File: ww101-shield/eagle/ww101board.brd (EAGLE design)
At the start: 64.8 x 73.3 mm, 66 parts, among them J6 U8G-096-OLED, J7 0, U7 CY8C4A45-48

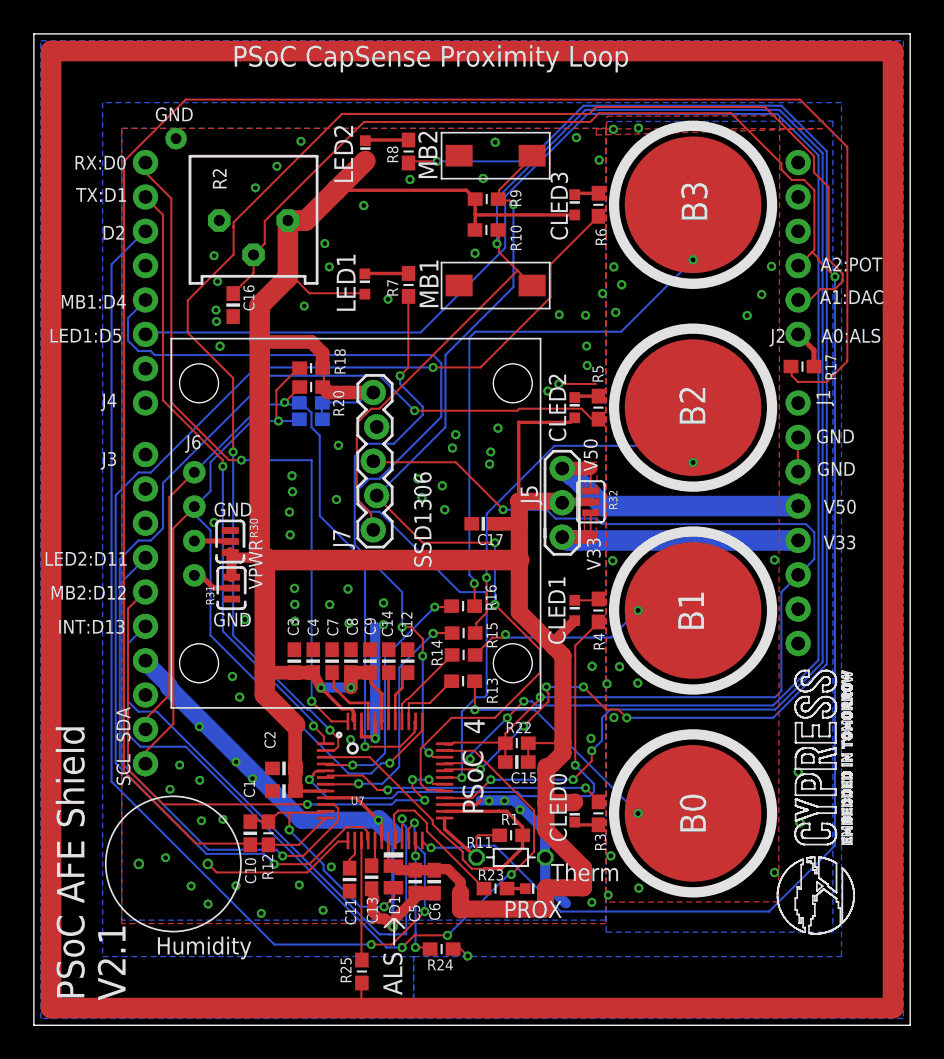
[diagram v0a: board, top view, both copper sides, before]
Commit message: a bunch of updates
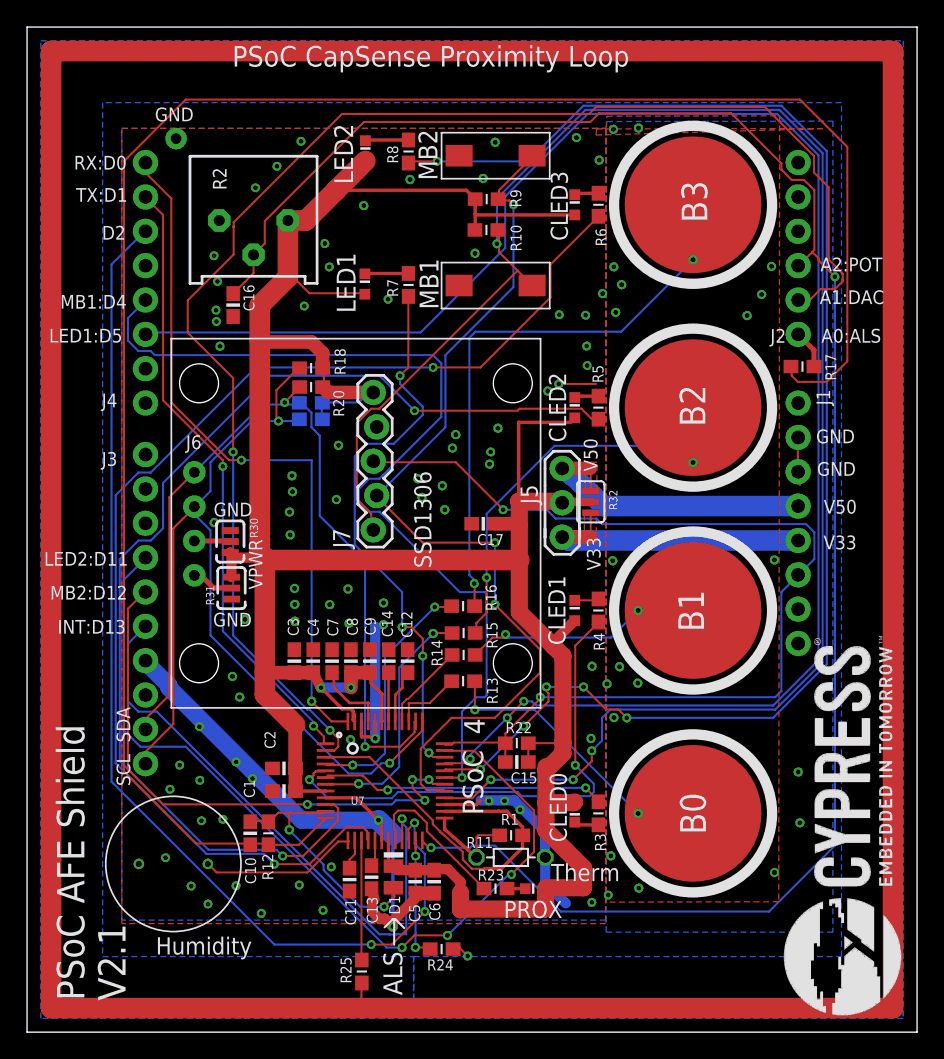
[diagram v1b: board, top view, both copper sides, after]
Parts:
- removed U$3: (no value), IOTExpert:CYPRESSLOGO
- added U$7: CYLOGO-SILK, ww101board:CYLOGO-SILK
- R18, R19, R20, R21: value 4.7K -> DNP
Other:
- board size 64.8 x 73.3 mm -> 65.8 x 74.3 mm
- board text added: "600-60500-01 REV2.1"
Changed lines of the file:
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@@
 <layer number="17" name="Pads" color="2" fill="1" visible="yes" active="yes"/>
 <layer number="18" name="Vias" color="2" fill="1" visible="yes" active="yes"/>
-<layer number="19" name="Unrouted" color="6" fill="1" visible="yes" active="yes"/>
-<layer number="20" name="Dimension" color="15" fill="1" visible="yes" active="yes"/>
+<layer number="19" name="Unrouted" color="6" fill="1" visible="no" active="yes"/>
+<layer number="20" name="Dimension" color="15" fill="1" visible="no" active="yes"/>
 <layer number="21" name="tPlace" color="7" fill="1" visible="yes" active="yes"/>
 <layer number="22" name="bPlace" color="7" fill="1" visible="yes" active="yes"/>
@@
 <board>
 <plain>
-<wire x1="-5.7404" y1="-9.1694" x2="59.055" y2="-9.1694" width="0" layer="20"/>
-<wire x1="59.055" y1="-9.1694" x2="59.055" y2="64.135" width="0" layer="20"/>
-<wire x1="59.055" y1="64.135" x2="-5.7404" y2="64.135" width="0" layer="20"/>
-<wire x1="-5.7404" y1="64.135" x2="-5.7404" y2="-9.1694" width="0" layer="20"/>
+<wire x1="-6.2484" y1="-9.6774" x2="59.563" y2="-9.6774" width="0" layer="20"/>
+<wire x1="59.563" y1="-9.6774" x2="59.563" y2="64.643" width="0" layer="20"/>
+<wire x1="59.563" y1="64.643" x2="-6.2484" y2="64.643" width="0" layer="20"/>
+<wire x1="-6.2484" y1="64.643" x2="-6.2484" y2="-9.6774" width="0" layer="20"/>
 <text x="36.164521875" y="24.462740625" size="1.016" layer="25" font="vector" ratio="15" rot="R90">V33</text>
 <text x="55.095140625" y="27.040840625" size="1.016" layer="25" font="vector" ratio="15" rot="R180">V33</text>
@@
 <wire x1="20.7797375" y1="-1.33858125" x2="20.99818125" y2="-1.33858125" width="0.1524" layer="21"/>
 <wire x1="20.99818125" y1="-1.33858125" x2="21.638259375" y2="-1.978659375" width="0.1524" layer="21"/>
+<text x="17.266921875" y="-7.929884375" size="1.27" layer="26" ratio="10" rot="MR0">600-60500-01 REV2.1</text>
 </plain>
 <attributes>
@@
 <attribute name="VALUE" x="21.5138" y="16.2306" size="0.6096" layer="27" font="vector" ratio="15" rot="R90" align="top-left"/>
 </element>
-<element name="R18" library="ww101board" package="0603-RES" value="4.7K" x="14.7574" y="39.4208" smashed="yes">
+<element name="R18" library="ww101board" package="0603-RES" value="DNP" x="14.7574" y="39.4208" smashed="yes">
 <attribute name="NAME" x="16.494759375" y="40.8914625" size="0.8128" layer="25" font="vector" ratio="15" rot="R270"/>
 <attribute name="VALUE" x="13.2334" y="37.7698" size="0.6096" layer="27" font="vector" ratio="15"/>
 </element>
-<element name="R19" library="ww101board" package="0603-RES" value="4.7K" x="14.732" y="35.6362" locked="yes" smashed="yes" rot="MR180">
+<element name="R19" library="ww101board" package="0603-RES" value="DNP" x="14.732" y="35.6362" locked="yes" smashed="yes" rot="MR180">
 <attribute name="NAME" x="10.7188" y="35.8902" size="0.8128" layer="26" font="vector" ratio="15" rot="MR180"/>
 <attribute name="VALUE" x="13.208" y="37.2872" size="0.6096" layer="28" font="vector" ratio="15" rot="MR180"/>
 </element>
-<element name="R20" library="ww101board" package="0603-RES" value="4.7K" x="14.7574" y="38.0238" locked="yes" smashed="yes">
+<element name="R20" library="ww101board" package="0603-RES" value="DNP" x="14.7574" y="38.0238" locked="yes" smashed="yes">
 <attribute name="NAME" x="17.205959375" y="35.829240625" size="0.8128" layer="25" font="vector" ratio="15" rot="R90"/>
 <attribute name="VALUE" x="13.2334" y="36.3728" size="0.6096" layer="27" font="vector" ratio="15"/>
 </element>
-<element name="R21" library="ww101board" package="0603-RES" value="4.7K" x="14.732" y="36.8554" locked="yes" smashed="yes" rot="MR180">
+<element name="R21" library="ww101board" package="0603-RES" value="DNP" x="14.732" y="36.8554" locked="yes" smashed="yes" rot="MR180">
 <attribute name="NAME" x="10.6426" y="37.1856" size="0.8128" layer="26" font="vector" ratio="15" rot="MR180"/>
 <attribute name="VALUE" x="13.208" y="38.5064" size="0.6096" layer="28" font="vector" ratio="15" rot="MR180"/>
 </element>
 <element name="U$1" library="ww101board" package="UNO_R3_SHIELD_NOLABELS" value="ARDUINO_R3_SHIELDNOLABELS" x="-0.03" y="0.01" locked="yes"/>
-<element name="U$3" library="IOTExpert" package="CYPRESSLOGO" value="" x="52.0573" y="7.2009" rot="R90"/>
 <element name="R22" library="ww101board" package="0603-RES" value="10K" x="29.96691875" y="11.69161875" smashed="yes" rot="R180">
 <attribute name="NAME" x="31.1023" y="13.243559375" size="0.8128" layer="25" font="vector" ratio="15" rot="R180"/>
@@
 <attribute name="VALUE" x="37.337996875" y="28.26511875" size="0.6096" layer="27" font="vector" ratio="15" rot="R90"/>
 </element>
+<element name="U$7" library="ww101board" package="CYLOGO-SILK" value="CYLOGO-SILK" x="58.399678125" y="-8.453115625" rot="R90"/>
 </elements>
 <signals>
